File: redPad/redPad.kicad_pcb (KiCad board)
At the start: 2 copper layers, 33 parts, among them J1 OLED_128x32, SW1 RotaryEncoder_Switch, SW2 RotaryEncoder_Switch, SW3 SW_Push, SW4 Switch

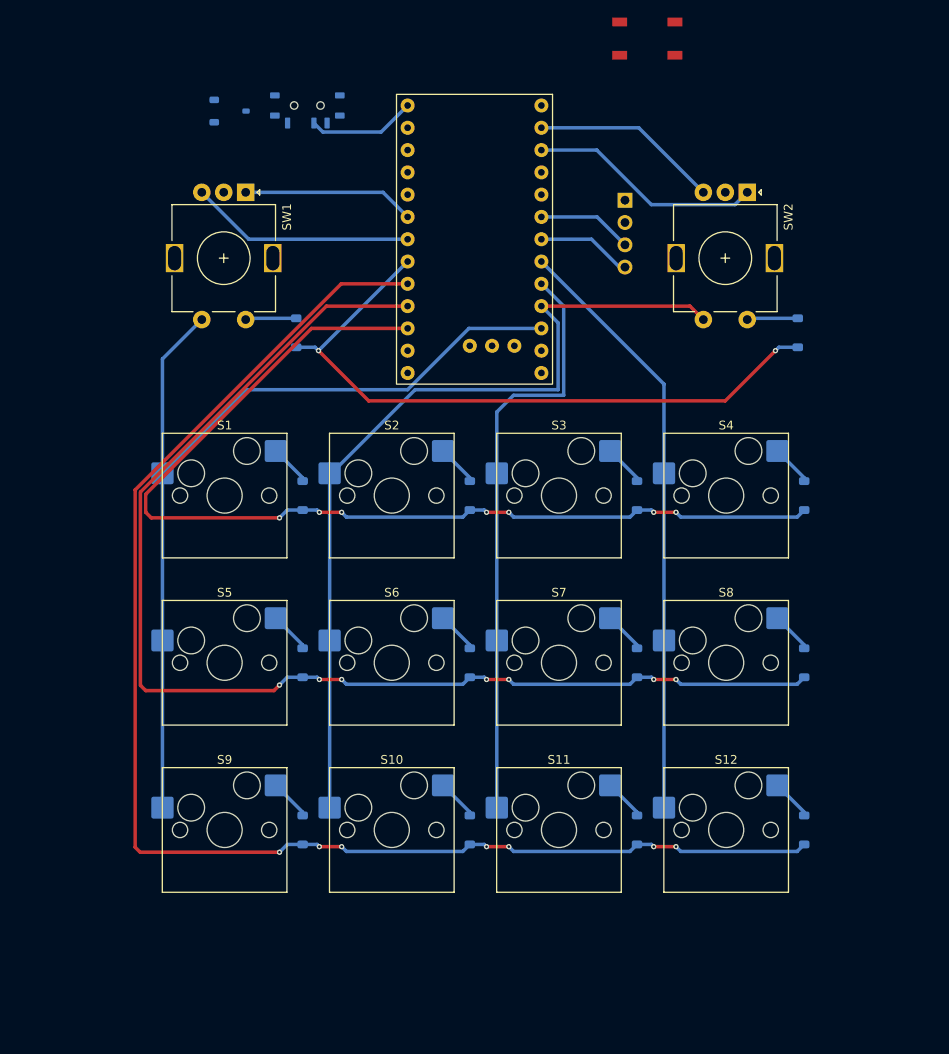
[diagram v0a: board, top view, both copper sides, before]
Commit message: Version 1.0 finalizada
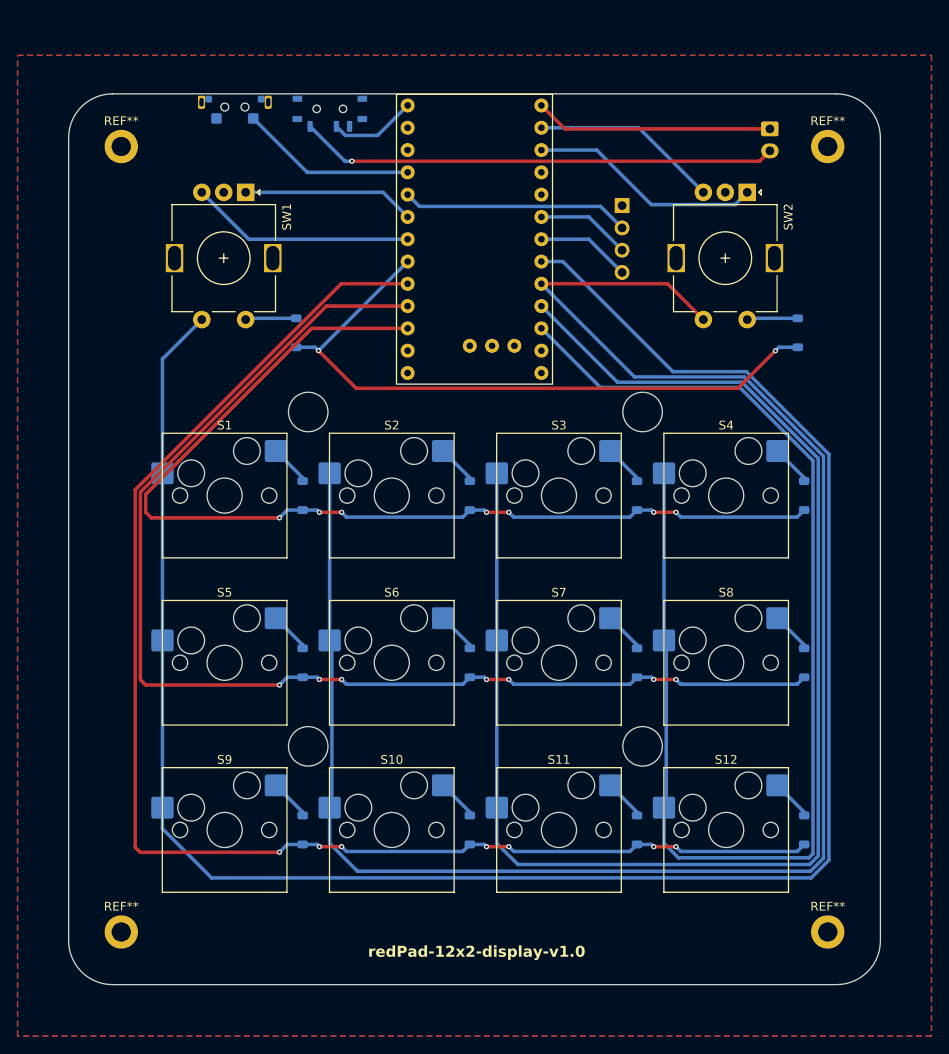
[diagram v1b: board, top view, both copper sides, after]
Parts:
- added REF**: MountingHole_2.2mm_M2_DIN965_Pad, MountingHole:MountingHole_2.2mm_M2_DIN965_Pad, F.Cu at (118.5, 122.8)
- added REF**: MountingHole_4.5mm, RedComponents:MountingHole_4.5mm, F.Cu at (177.9, 63.5)
- added REF**: MountingHole_2.2mm_M2_DIN965_Pad, MountingHole:MountingHole_2.2mm_M2_DIN965_Pad, F.Cu at (199.0, 33.2)
- added REF**: MountingHole_2.2mm_M2_DIN965_Pad, MountingHole:MountingHole_2.2mm_M2_DIN965_Pad, F.Cu at (118.5, 33.2)
- added REF**: MountingHole_4.5mm, RedComponents:MountingHole_4.5mm, F.Cu at (177.9, 101.6)
- added REF**: MountingHole_4.5mm, RedComponents:MountingHole_4.5mm, F.Cu at (139.8, 63.5)
- added REF**: MountingHole_2.2mm_M2_DIN965_Pad, MountingHole:MountingHole_2.2mm_M2_DIN965_Pad, F.Cu at (199.0, 122.8)
- added REF**: MountingHole_4.5mm, RedComponents:MountingHole_4.5mm, F.Cu at (139.8, 101.6)
- BT1: footprint Connector_JST:JST_ACH_BM01B-ACHSS-A-GAN-ETF_1x01-1MP_P1.20mm_Vertical -> Connector_JST:JST_EH_S2B-EH_1x02_P2.50mm_Horizontal
- SW3: footprint ScottoKeebs_Components:Button_TL3342 -> RedComponents:SW TS-B003-Y; moved to B.Cu
- moved BT1 61.6 mm to (192.4, 31.2), turned to -90 degrees
- moved SW3 47.6 mm to (131.4, 28.8)
- moved SW4 2.59 mm to (142.3, 29.0)
- moved J1 0.70 mm to (177.2, 49.8)
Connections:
- BT1 pad 1: Net-(BT1-+) -> BAT -
- SW4 pad 1: Net-(BT1-+) -> Net-(BT1--)
- SuperMini-NRF1 pad 10: COL 1 -> COL 2
- SuperMini-NRF1 pad 11: COL 0 -> COL 3
- SuperMini-NRF1 pad 8: COL 3 -> COL 0
- SuperMini-NRF1 pad 9: COL 2 -> COL 1
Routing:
- net COL 0: track 107.5 -> 227.1 mm
- net COL 1: track 97.5 -> 207.0 mm
- net COL 2: track 67.2 -> 164.2 mm
- net COL 3: track 68.0 -> 142.6 mm
- net Net-(BT1--): track 0.00 -> 54.5 mm, vias 0 -> 1
- net BAT -: track 0.00 -> 27.1 mm
- net VCC: track 0.00 -> 26.0 mm
- net RST: track 0.00 -> 20.1 mm
- net BAT +: track 12.4 -> 9.95 mm
- net ROW 3: track 76.6 -> 75.4 mm
- net ROW 1: track 139.8 -> 138.9 mm
- net OLED SDA: track 11.0 -> 11.6 mm
- added copper zone on B.Cu, net GND
- added copper zone on F.Cu, net GND
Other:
- board outline added: 92.5 x 101.5 mm
- board text added: "redPad-12x2-display-v1.0"
